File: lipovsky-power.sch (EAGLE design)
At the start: 97 parts, among them J1 M04-929J, J2 M04-929J, J3 M04-929J, J4 M04-929J, Q1 NMOS30V_30A, Q12 NMOS40V_10A, Q14 NMOS40V_10A, Q16 NMOS40V_10A, Q18 NMOS40V_10A, Q2 2NMOS30V_0.1A, Q21 PMOS30V_11A, Q22 PMOS30V_11A, Q23 NMOS40V_10A, Q24 NMOS40V_10A, Q25 PMOS30V_11A, Q26 PMOS30V_11A, Q27 NMOS40V_10A, Q28 NMOS40V_10A, Q3 2PMOS50V_0.17A, Q31 PMOS30V_11A, Q32 PMOS30V_11A, Q33 PMOS30V_11A, Q34 PMOS30V_11A, Q35 PMOS30V_11A, Q36 PMOS30V_11A, Q37 PMOS30V_11A, Q38 PMOS30V_11A, Q4 2PMOS50V_0.17A, Q41 PMOS30V_11A, Q42 PMOS30V_11A, Q43 PMOS30V_11A, Q44 PMOS30V_11A, Q45 PMOS30V_11A, Q46 PMOS30V_11A, Q47 PMOS30V_11A, Q48 PMOS30V_11A, Q5 2NMOS30V_0.1A, Q51 PMOS30V_11A, Q52 PMOS30V_11A, Q53 PMOS30V_11A, Q54 PMOS30V_11A, Q55 PMOS30V_11A, Q56 PMOS30V_11A, Q57 PMOS30V_11A, Q58 PMOS30V_11A, Q62 PMOS30V_11A, Q64 PMOS30V_11A, Q66 PMOS30V_11A, Q68 PMOS30V_11A, T1 TFORM_4_4311_4A4, U1 DG508BEN-T1-GE4, U2 DG508BEN-T1-GE4, U3 74HC595, U4 LTC3805-5IDD, U6 AR30N60PPA-13

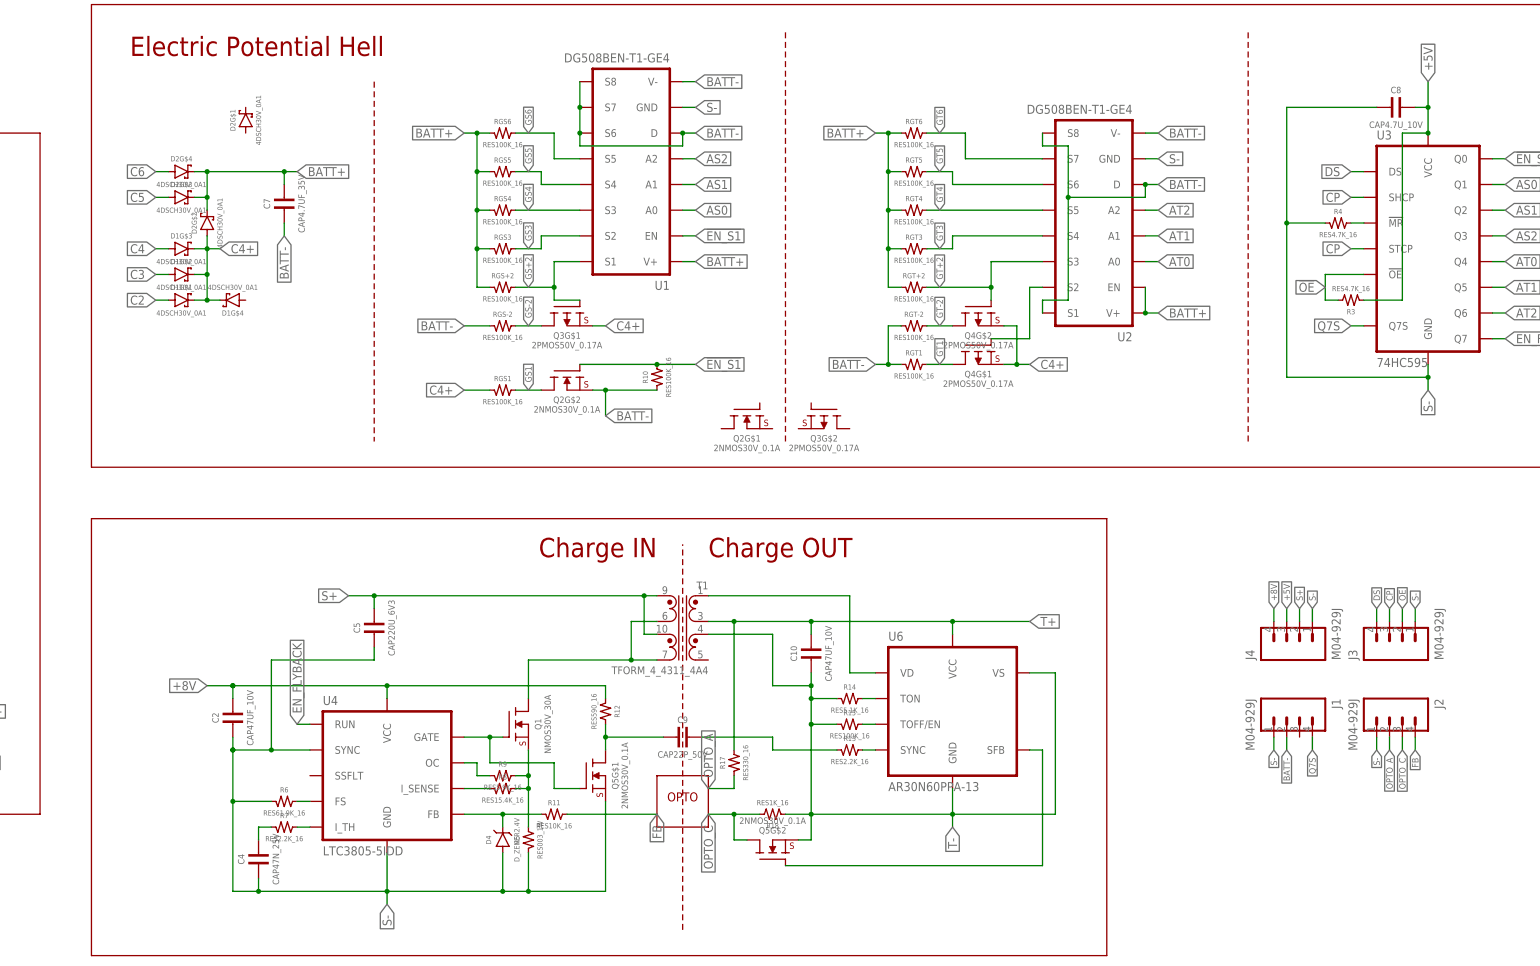
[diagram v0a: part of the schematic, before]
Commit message: .
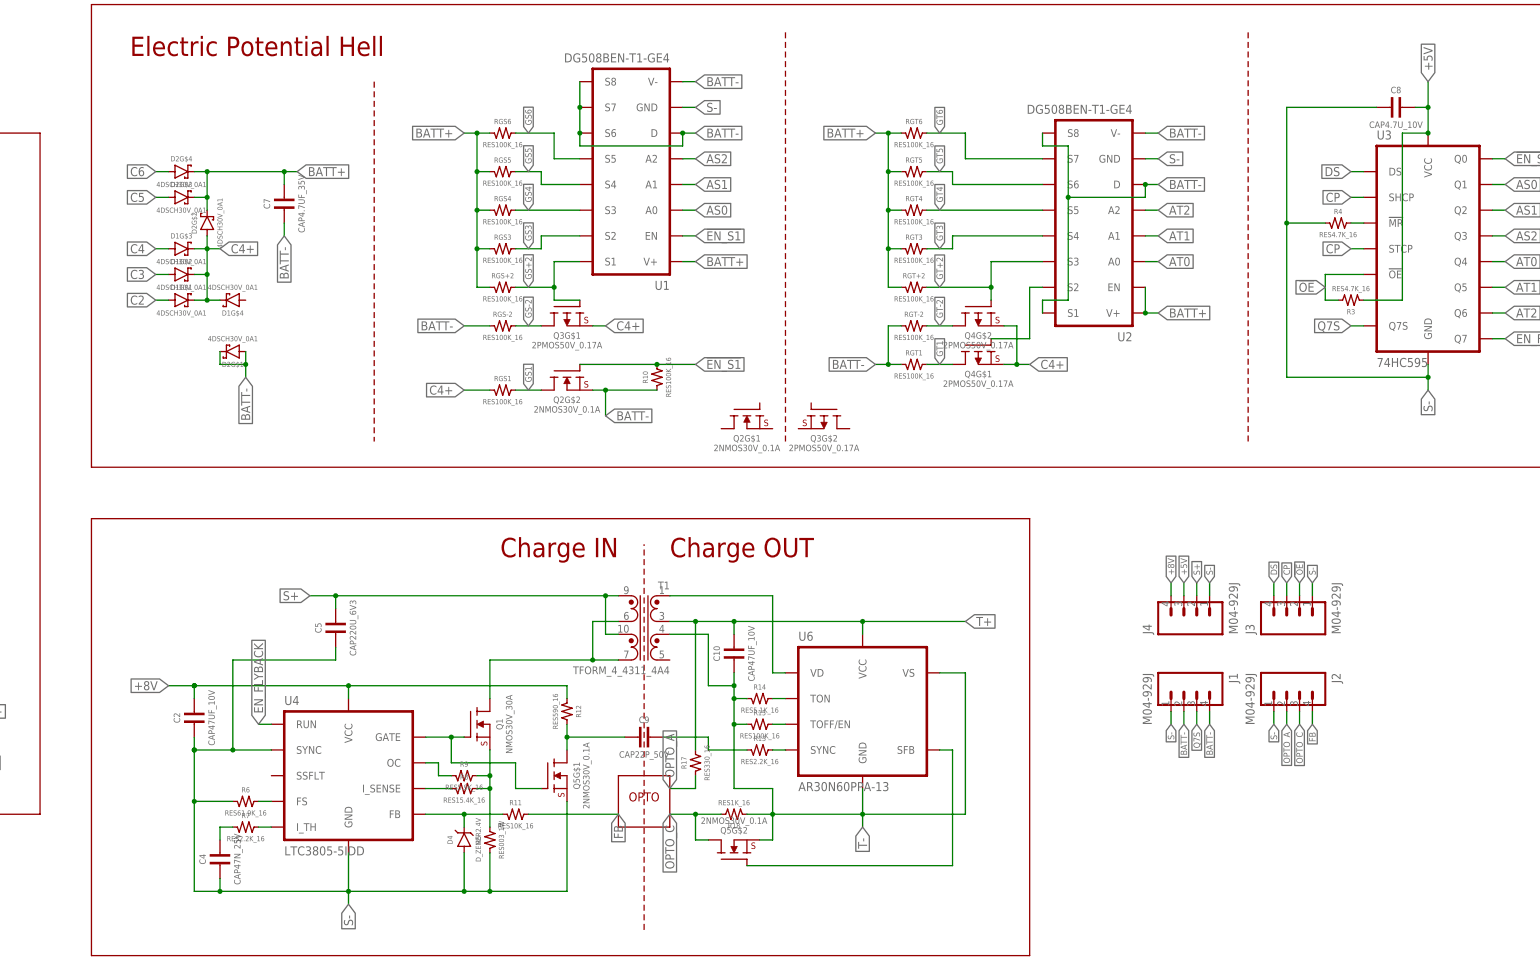
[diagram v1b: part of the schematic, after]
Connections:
- net BATT-: now also D2G$1.A, D2G$1.C, J1.4
- net Q7S: now also J1.3; no longer J1.4
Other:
- moved on the sheet: C10, C2, C4, C5, C9, D2G$1, D4, J1, J2, J3, J4, Q1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
